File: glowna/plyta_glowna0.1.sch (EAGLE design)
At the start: 111 parts, among them IC1 4504D, Q1 CSM-7X-DU, Q2 N-HEXFET-2D_SOT232-IRLL014N, Q3 N-HEXFET-2D_SOT232-IRLL014N, Q4 N-HEXFET-2D_SOT232-IRLL014N, Q5 N-HEXFET-2D_SOT232-IRLL014N, Q6 N-HEXFET-2D_SOT232-IRLL014N, X1 MINI-USB_SHIELD5P2-32005-601

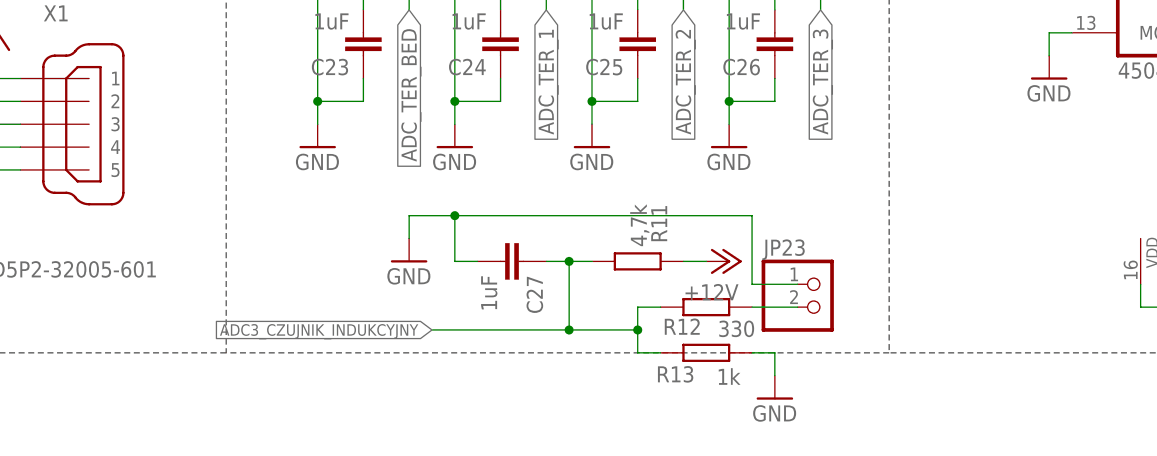
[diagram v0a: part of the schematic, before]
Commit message: indukcyjne
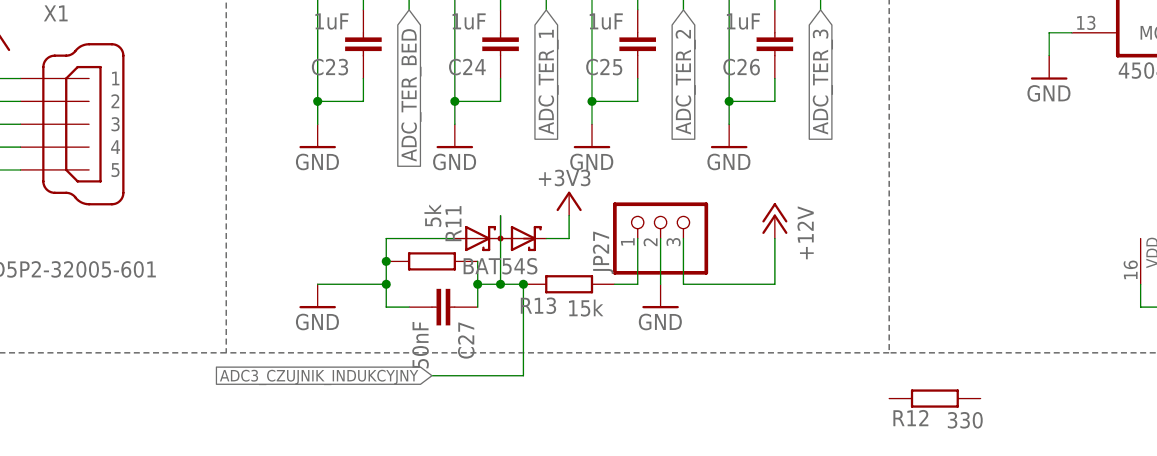
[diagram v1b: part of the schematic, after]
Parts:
- removed JP23: (no value), pinhead:PINHD-1X2
- added D8: BAT54S, diode:BAT54S
- added JP27: (no value), pinhead:PINHD-1X3
- C27: value 1uF -> 50nF
- R11: value 4,7k -> 5k
- R13: value 1k -> 15k
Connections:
- removed net N$16: JP23.2, R12.1
- new net N$38: JP27.1, R13.2
- net +12V: now also JP27.3; no longer R11.1
- net +3V3: now also D8.C2
- net ADC3_CZUJNIK_INDUKCYJNY: now also D8.C1A2, R11.1; no longer R11.2, R12.2
- net GND: now also D8.A1, JP27.2, R11.2; no longer R13.2
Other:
- moved on the sheet: C27, R11, R12, R13
